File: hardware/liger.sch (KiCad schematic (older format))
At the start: 39 parts, among them U1? SPX3819

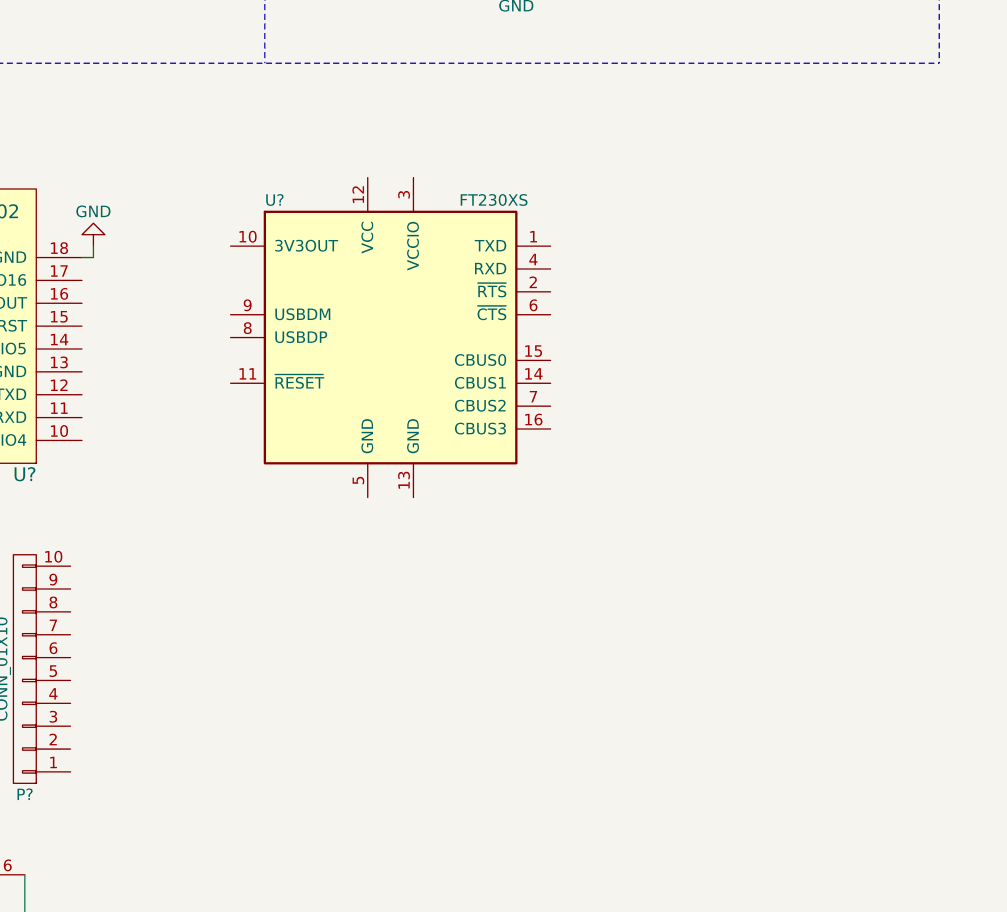
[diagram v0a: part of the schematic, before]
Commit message: update
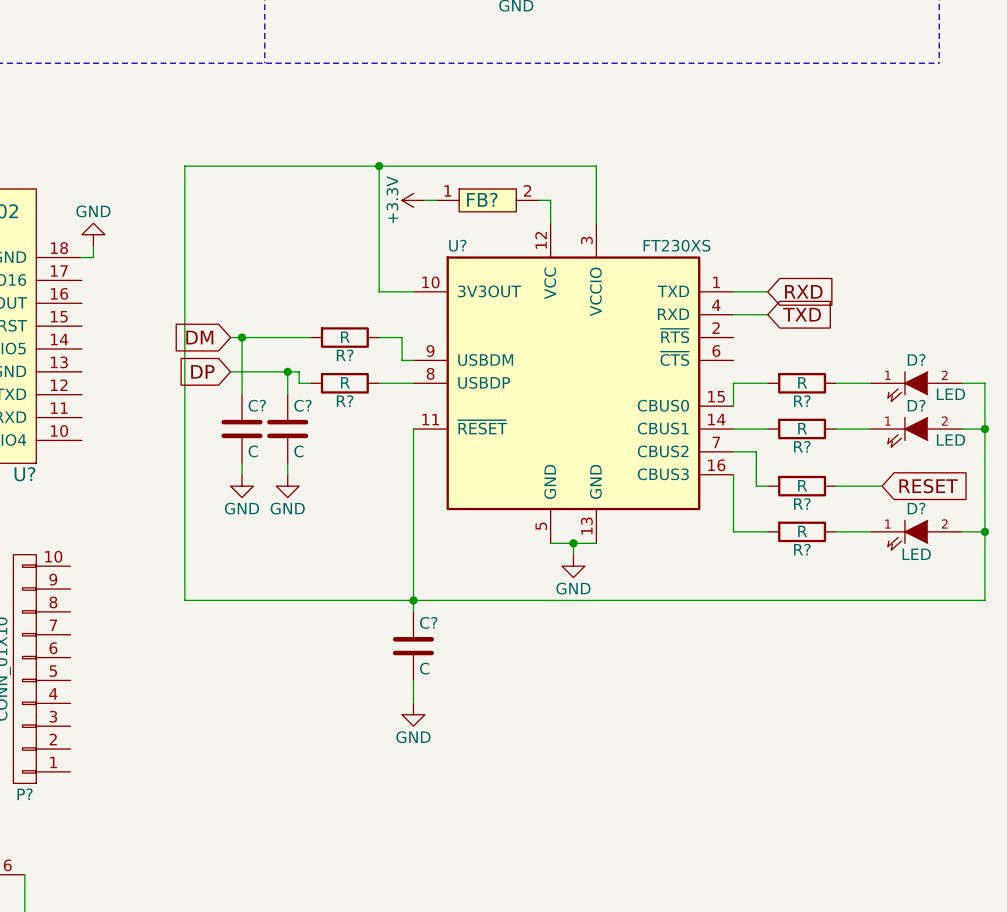
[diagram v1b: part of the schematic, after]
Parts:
- added C? (x3): C, symbol C
- added D? (x3): LED, symbol LED
- added FB?: BK0603HS330-T, symbol BK0603HS330-T
- added R? (x6): R, symbol R
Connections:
- net +3V3: now also FB?.1
- net DM: now also C?.1, R?.2
- net DP: now also C?.1, R?.2
- net GND: now also U?.13 (GND), U?.5 (GND), C?.2, C?.2, C?.2
- net RXD: now reaches U?.1 (TXD)
- net at U?.10 (3V3OUT): now also U?.11 (~RESET), U?.3 (VCCIO), C?.1, D?.2 (A), D?.2 (A), D?.2 (A)
- net at U?.12 (VCC): now also FB?.2
- net at U?.14 (CBUS1): now also R?.2
- net at U?.15 (CBUS0): now also R?.2
- net at U?.16 (CBUS3): now also R?.2
- net TXD: now reaches U?.4 (RXD)
- net at U?.7 (CBUS2): now also R?.2
- net at U?.8 (USBDP): now also R?.1
- net at U?.9 (USBDM): now also R?.1
- new net: D?.1 (K), R?.1 (x3)
- new net RESET: R?.1
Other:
- moved on the sheet: U?
